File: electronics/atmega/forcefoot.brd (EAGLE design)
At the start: 60 x 43.6 mm, 71 parts, among them U2 ATMEGA168

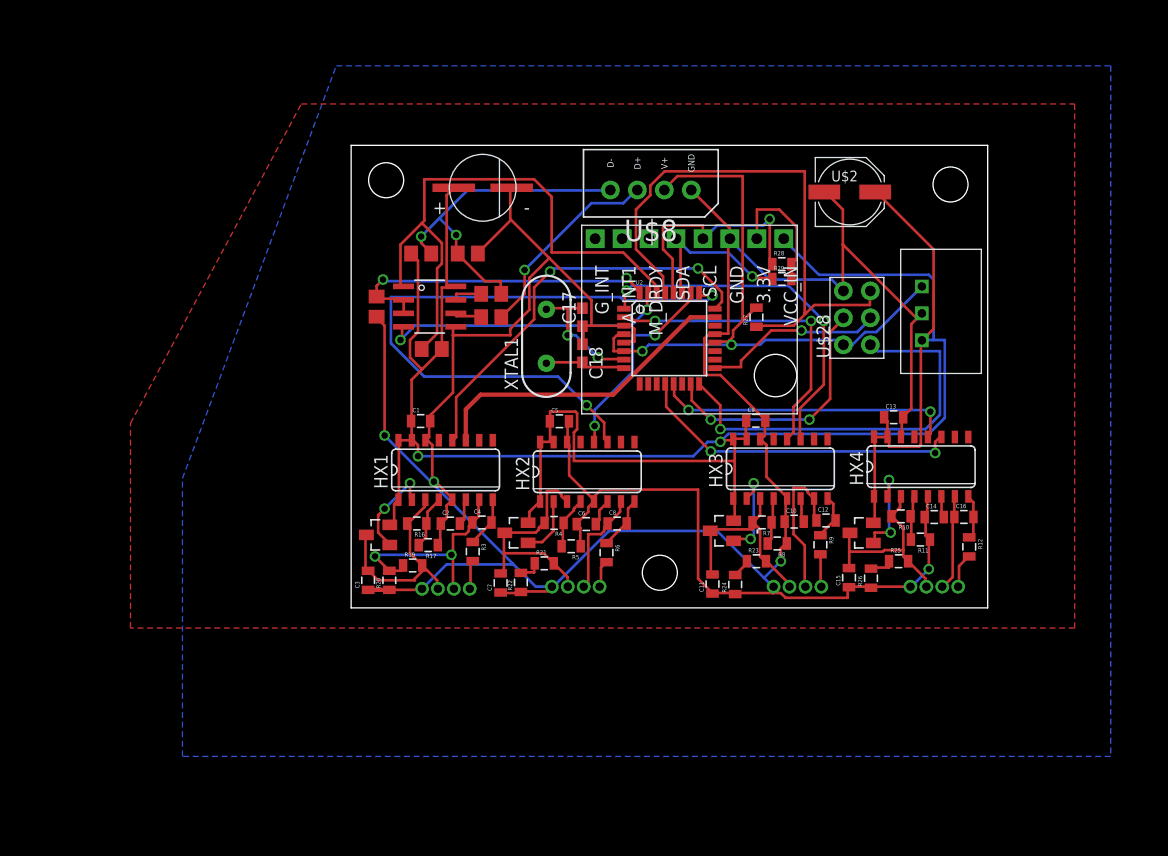
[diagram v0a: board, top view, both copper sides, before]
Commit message: Board fixes
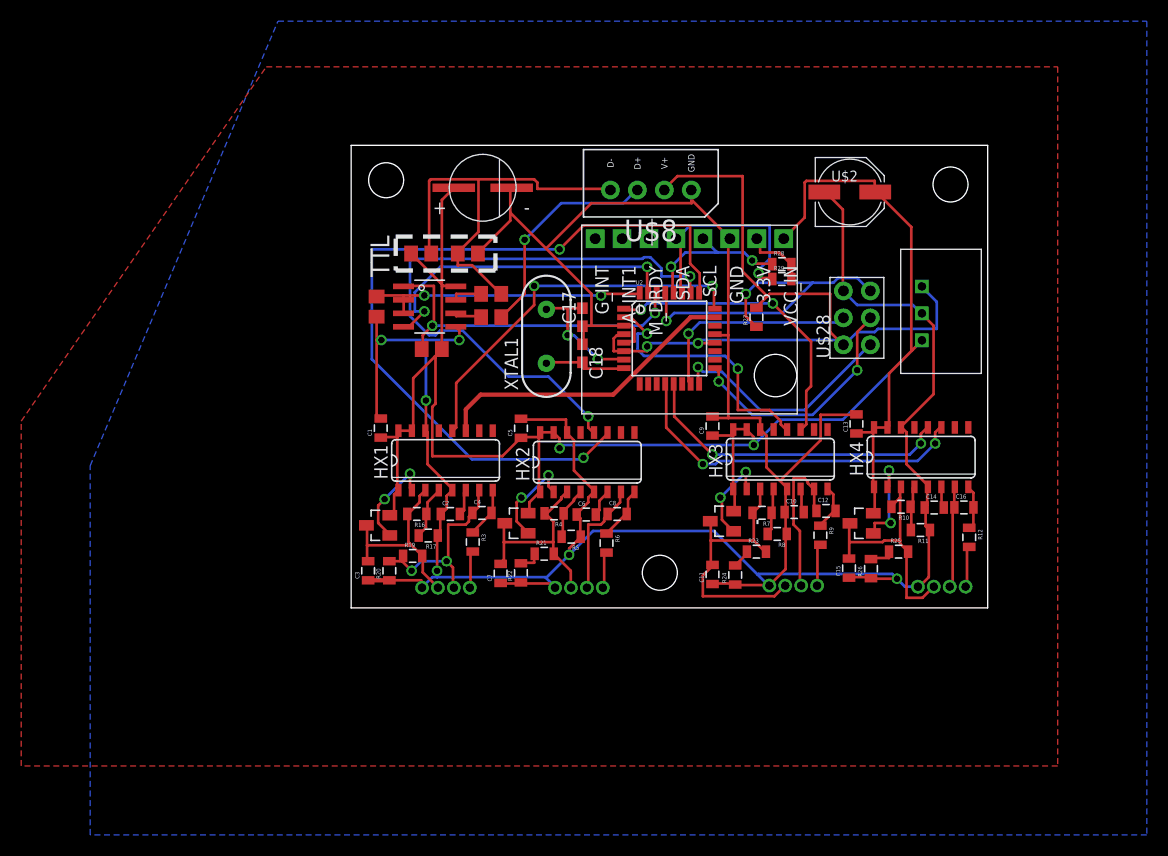
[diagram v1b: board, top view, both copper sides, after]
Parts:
- moved C9 4.11 mm to (34.1, 16.9), turned to 90 degrees
- moved C1 3.82 mm to (2.79, 16.8), turned to 90 degrees
- moved C5 3.68 mm to (16.0, 16.7), turned to 90 degrees
- moved C13 3.57 mm to (47.6, 17.1), turned to 90 degrees
- moved R4 0.90 mm to (19.1, 8.71)
- moved C10 0.90 mm to (41.8, 8.83)
- moved C11 0.90 mm to (34.1, 2.95)
- moved C12 0.90 mm to (44.8, 8.94)
- moved C14 0.90 mm to (55.0, 9.26)
- moved C16 0.90 mm to (57.8, 9.27)
- moved C2 0.90 mm to (9.35, 8.65)
- moved C4 0.90 mm to (12.3, 8.75)
- moved C8 0.90 mm to (25.1, 8.65)
- moved HX3 0.90 mm to (40.5, 13.8)
- moved HX4 0.90 mm to (53.7, 14.0)
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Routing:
- net VCC: track 222.3 -> 176.6 mm
- net DOUT2: track 19.1 -> 57.5 mm
- net RX: track 54.4 -> 32.8 mm, vias 0 -> 2
- net RESET: track 53.3 -> 34.4 mm, vias 0 -> 2
- net MISO: track 39.2 -> 22.1 mm
- net GND: track 303.7 -> 290.0 mm, vias 4 -> 6
- net SCK2: track 61.6 -> 75.3 mm
- net VIN: track 62.0 -> 73.6 mm
- net IMU_SCL: track 23.1 -> 15.1 mm, vias 1 -> 2
- net AVDD$3: track 19.1 -> 26.6 mm
- net RS-: track 32.1 -> 39.0 mm, vias 2 -> 0
- net 3.3: track 12.3 -> 6.25 mm
- net SCK3: track 34.1 -> 28.1 mm
- net SCK: track 17.2 -> 22.9 mm, vias 1 -> 2
- net IMU_SDA: track 16.1 -> 21.4 mm
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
